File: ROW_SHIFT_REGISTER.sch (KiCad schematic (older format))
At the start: 23 parts, among them Q12 AO3407A, Q13 SSM3K35AMFV, Q14 SSM3K35AMFV, U10 74HC595, U11 74HC595, U12 74HC595, U9 74HC595

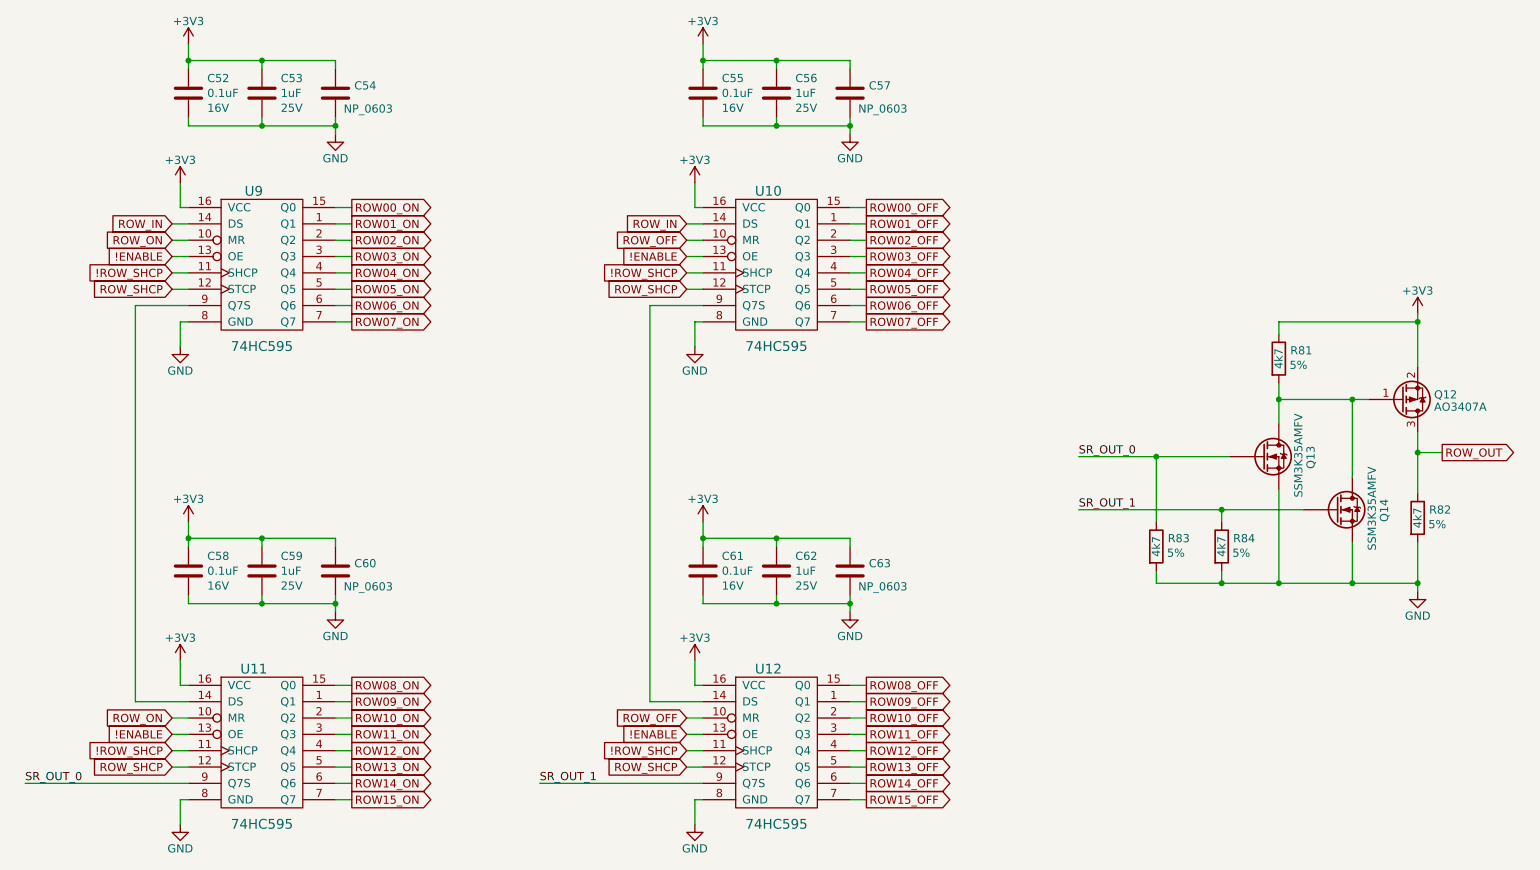
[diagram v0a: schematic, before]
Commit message: automated commit
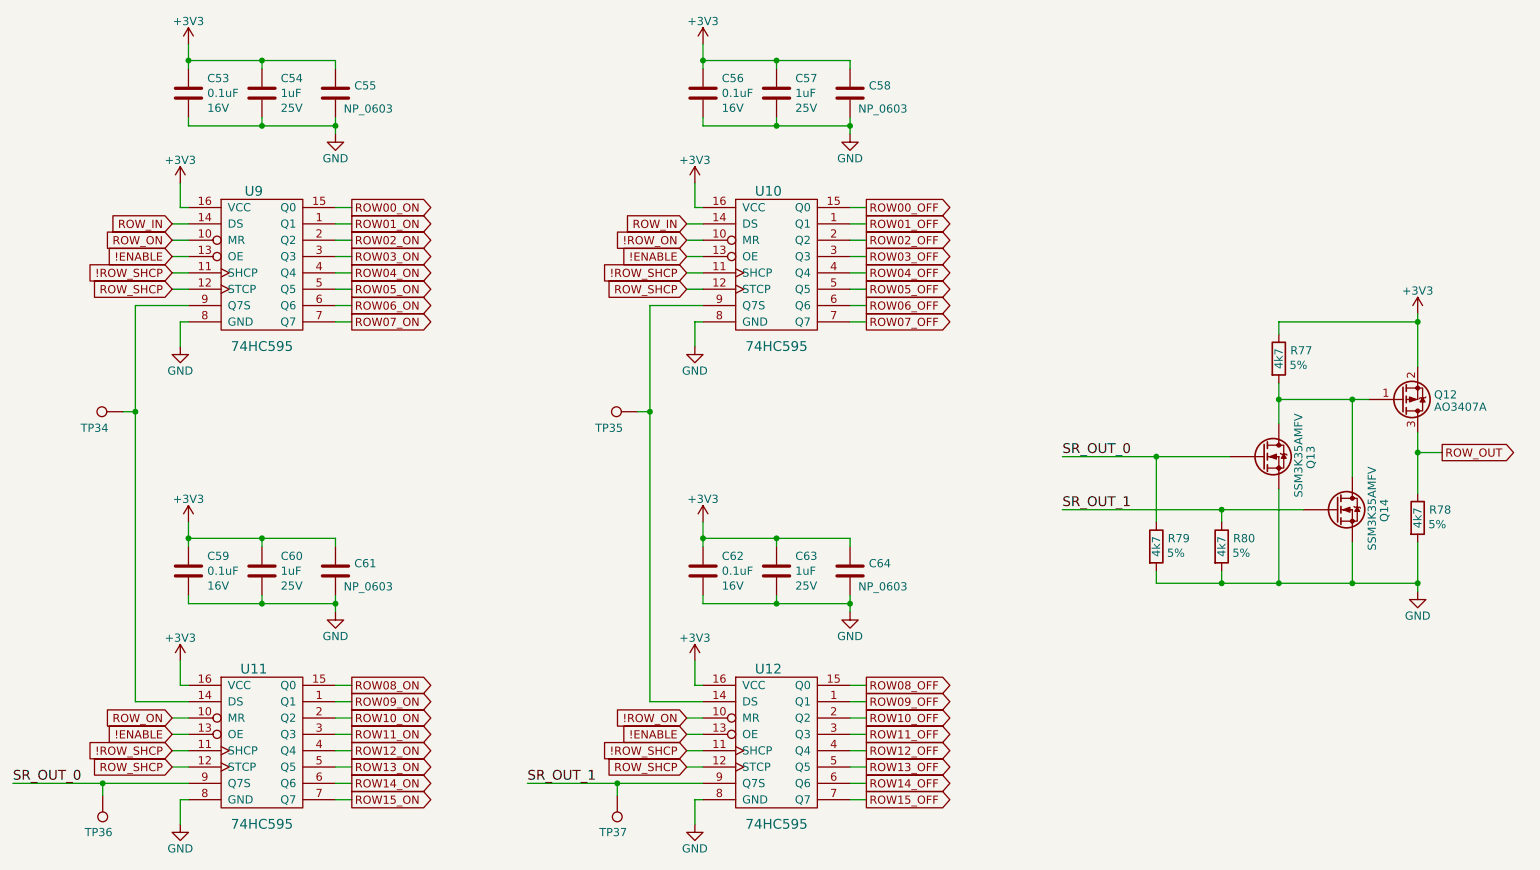
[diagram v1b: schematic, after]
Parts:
- added TP34, TP35, TP36, TP37: TestPoint, symbol Connector:TestPoint
- renumbered C52 to C53, C53 to C54, C54 to C55, C55 to C56, C56 to C57, C57 to C58, C58 to C59, C59 to C60, C60 to C61, C61 to C62, C62 to C63, C63 to C64, R81 to R77, R82 to R78, R83 to R79, R84 to R80
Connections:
- net SR_OUT_0: now also TP36.1
- net SR_OUT_1: now also TP37.1
- net at U11.14 (DS), U9.9 (Q7S): now also TP34.1
- net at U10.9 (Q7S), U12.14 (DS): now also TP35.1
- net ROW_OFF renamed !ROW_ON
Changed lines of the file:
@@
 	1925 2850 1600 2850
 Wire Wire Line
-	1600 2850 1600 5275
+	1600 2850 1600 3500
 Wire Wire Line
 	1600 5275 1925 5275
 Wire Wire Line
-	1925 2350 1825 2350
-Wire Wire Line
 	5025 2100 5025 2250
 Wire Wire Line
@@
 Wire Wire Line
 	5075 2850 4750 2850
-Wire Wire Line
-	4750 2850 4750 5275
 Wire Wire Line
 	4750 5275 5075 5275
@@
 P 2375 1550
 AR Path="/622B9EDC" Ref="C?"  Part="1"
-AR Path="/621F0CB4/622B9EDC" Ref="C53"  Part="1"
-F 0 "C53" H 2490 1641 50  0000 L CNN
+AR Path="/621F0CB4/622B9EDC" Ref="C54"  Part="1"
+F 0 "C54" H 2490 1641 50  0000 L CNN
 F 1 "CL10B105KA8NNNC" H 1425 1100 50  0001 L BNN
 F 2 "Capacitor_SMD:C_0603_1608Metric" H 1425 1000 50  0001 L BNN
@@
 P 1925 1550
 AR Path="/622B9EE4" Ref="C?"  Part="1"
-AR Path="/621F0CB4/622B9EE4" Ref="C52"  Part="1"
-F 0 "C52" H 2040 1641 50  0000 L CNN
+AR Path="/621F0CB4/622B9EE4" Ref="C53"  Part="1"
+F 0 "C53" H 2040 1641 50  0000 L CNN
 F 1 "CL10B104KO8NNNC" H 975 1100 50  0001 L BNN
 F 2 "Capacitor_SMD:C_0603_1608Metric" H 975 1000 50  0001 L BNN
@@
 P 2825 1550
 AR Path="/622B9EEB" Ref="C?"  Part="1"
-AR Path="/621F0CB4/622B9EEB" Ref="C54"  Part="1"
-F 0 "C54" H 2940 1596 50  0000 L CNN
+AR Path="/621F0CB4/622B9EEB" Ref="C55"  Part="1"
+F 0 "C55" H 2940 1596 50  0000 L CNN
 F 1 "NP_0603" H 2875 1425 50  0000 L BNN
 F 2 "Capacitor_SMD:C_0603_1608Metric" H 1875 1000 50  0001 L BNN
@@
 P 2375 4475
 AR Path="/622B9F13" Ref="C?"  Part="1"
-AR Path="/621F0CB4/622B9F13" Ref="C59"  Part="1"
-F 0 "C59" H 2490 4566 50  0000 L CNN
+AR Path="/621F0CB4/622B9F13" Ref="C60"  Part="1"
+F 0 "C60" H 2490 4566 50  0000 L CNN
 F 1 "CL10B105KA8NNNC" H 1425 4025 50  0001 L BNN
 F 2 "Capacitor_SMD:C_0603_1608Metric" H 1425 3925 50  0001 L BNN
@@
 P 1925 4475
 AR Path="/622B9F1B" Ref="C?"  Part="1"
-AR Path="/621F0CB4/622B9F1B" Ref="C58"  Part="1"
-F 0 "C58" H 2040 4566 50  0000 L CNN
+AR Path="/621F0CB4/622B9F1B" Ref="C59"  Part="1"
+F 0 "C59" H 2040 4566 50  0000 L CNN
 F 1 "CL10B104KO8NNNC" H 975 4025 50  0001 L BNN
 F 2 "Capacitor_SMD:C_0603_1608Metric" H 975 3925 50  0001 L BNN
@@
 P 5525 1550
 AR Path="/622B9F4A" Ref="C?"  Part="1"
-AR Path="/621F0CB4/622B9F4A" Ref="C56"  Part="1"
-F 0 "C56" H 5640 1641 50  0000 L CNN
+AR Path="/621F0CB4/622B9F4A" Ref="C57"  Part="1"
+F 0 "C57" H 5640 1641 50  0000 L CNN
 F 1 "CL10B105KA8NNNC" H 4575 1100 50  0001 L BNN
 F 2 "Capacitor_SMD:C_0603_1608Metric" H 4575 1000 50  0001 L BNN
@@
 P 5075 1550
 AR Path="/622B9F52" Ref="C?"  Part="1"
-AR Path="/621F0CB4/622B9F52" Ref="C55"  Part="1"
-F 0 "C55" H 5190 1641 50  0000 L CNN
+AR Path="/621F0CB4/622B9F52" Ref="C56"  Part="1"
+F 0 "C56" H 5190 1641 50  0000 L CNN
 F 1 "CL10B104KO8NNNC" H 4125 1100 50  0001 L BNN
 F 2 "Capacitor_SMD:C_0603_1608Metric" H 4125 1000 50  0001 L BNN
@@
 P 5525 4475
 AR Path="/622B9F81" Ref="C?"  Part="1"
-AR Path="/621F0CB4/622B9F81" Ref="C62"  Part="1"
-F 0 "C62" H 5640 4566 50  0000 L CNN
+AR Path="/621F0CB4/622B9F81" Ref="C63"  Part="1"
+F 0 "C63" H 5640 4566 50  0000 L CNN
 F 1 "CL10B105KA8NNNC" H 4575 4025 50  0001 L BNN
 F 2 "Capacitor_SMD:C_0603_1608Metric" H 4575 3925 50  0001 L BNN
@@
 P 5075 4475
 AR Path="/622B9F89" Ref="C?"  Part="1"
-AR Path="/621F0CB4/622B9F89" Ref="C61"  Part="1"
-F 0 "C61" H 5190 4566 50  0000 L CNN
+AR Path="/621F0CB4/622B9F89" Ref="C62"  Part="1"
+F 0 "C62" H 5190 4566 50  0000 L CNN
 F 1 "CL10B104KO8NNNC" H 4125 4025 50  0001 L BNN
 F 2 "Capacitor_SMD:C_0603_1608Metric" H 4125 3925 50  0001 L BNN
@@
 ROW_ON
 Text GLabel 4975 2450 0    50   Input ~ 0
-ROW_OFF
+!ROW_ON
 Text GLabel 4975 5375 0    50   Input ~ 0
-ROW_OFF
-Text Label 925  5775 0    50   ~ 0
+!ROW_ON
+Text Label 850  5775 0    60   ~ 0
 SR_OUT_0
-Wire Wire Line
-	925  5775 1925 5775
-Text Label 4075 5775 0    50   ~ 0
+Text Label 4000 5775 0    60   ~ 0
 SR_OUT_1
-Wire Wire Line
-	4075 5775 5075 5775
 $Comp
 L custom:SSM3K35AMFV Q?
@@
 	1    0    0    -1
 $EndComp
-Text Label 7375 4100 0    50   ~ 0
+Text Label 7275 4100 0    60   ~ 0
 SR_OUT_1
-Text Label 7375 3775 0    50   ~ 0
+Text Label 7275 3775 0    60   ~ 0
 SR_OUT_0
 Wire Wire Line
-	7375 3775 7850 3775
-$Comp
-L custom:CRG0603F4K7 R83
+	7275 3775 7850 3775
+$Comp
+L custom:CRG0603F4K7 R79
 U 1 1 5D1EAA64
 P 7850 4325
-F 0 "R83" H 7920 4345 50  0000 L BNN
+F 0 "R79" H 7920 4345 50  0000 L BNN
 F 1 "CRG0603F4K7" H 7150 3925 50  0001 L BNN
 F 2 "Resistor_SMD:R_0603_1608Metric" H 7150 3825 50  0001 L BNN
@@
 $EndComp
 $Comp
-L custom:CRG0603F4K7 R84
+L custom:CRG0603F4K7 R80
 U 1 1 5D1EB3B5
 P 8250 4325
-F 0 "R84" H 8320 4345 50  0000 L BNN
+F 0 "R80" H 8320 4345 50  0000 L BNN
 F 1 "CRG0603F4K7" H 7550 3925 50  0001 L BNN
 F 2 "Resistor_SMD:R_0603_1608Metric" H 7550 3825 50  0001 L BNN
@@
 	8600 4550 9050 4550
 $Comp
-L custom:CRG0603F4K7 R81
+L custom:CRG0603F4K7 R77
 U 1 1 5D2191D0
 P 8600 3175
-F 0 "R81" H 8670 3195 50  0000 L BNN
+F 0 "R77" H 8670 3195 50  0000 L BNN
 F 1 "CRG0603F4K7" H 7900 2775 50  0001 L BNN
 F 2 "Resistor_SMD:R_0603_1608Metric" H 7900 2675 50  0001 L BNN
@@
 	9050 3425 8600 3425
 $Comp
-L custom:CRG0603F4K7 R82
+L custom:CRG0603F4K7 R78
 U 1 1 5D22CE7A
 P 9450 4150
-F 0 "R82" H 9520 4170 50  0000 L BNN
+F 0 "R78" H 9520 4170 50  0000 L BNN
 F 1 "CRG0603F4K7" H 8750 3750 50  0001 L BNN
 F 2 "Resistor_SMD:R_0603_1608Metric" H 8750 3650 50  0001 L BNN
@@
 	7850 3775 8300 3775
 Wire Wire Line
-	7375 4100 8250 4100
+	7275 4100 8250 4100
 Wire Wire Line
 	7850 4550 8250 4550
@@
 P 2825 4475
 AR Path="/5D052A90" Ref="C?"  Part="1"
-AR Path="/621F0CB4/5D052A90" Ref="C60"  Part="1"
-F 0 "C60" H 2940 4521 50  0000 L CNN
+AR Path="/621F0CB4/5D052A90" Ref="C61"  Part="1"
+F 0 "C61" H 2940 4521 50  0000 L CNN
 F 1 "NP_0603" H 2875 4350 50  0000 L BNN
 F 2 "Capacitor_SMD:C_0603_1608Metric" H 1875 3925 50  0001 L BNN
@@
 P 5975 4475
 AR Path="/5D053185" Ref="C?"  Part="1"
-AR Path="/621F0CB4/5D053185" Ref="C63"  Part="1"
-F 0 "C63" H 6090 4521 50  0000 L CNN
+AR Path="/621F0CB4/5D053185" Ref="C64"  Part="1"
+F 0 "C64" H 6090 4521 50  0000 L CNN
 F 1 "NP_0603" H 6025 4350 50  0000 L BNN
 F 2 "Capacitor_SMD:C_0603_1608Metric" H 5025 3925 50  0001 L BNN
@@
 P 5975 1550
 AR Path="/5D053792" Ref="C?"  Part="1"
-AR Path="/621F0CB4/5D053792" Ref="C57"  Part="1"
-F 0 "C57" H 6090 1596 50  0000 L CNN
+AR Path="/621F0CB4/5D053792" Ref="C58"  Part="1"
+F 0 "C58" H 6090 1596 50  0000 L CNN
 F 1 "NP_0603" H 6025 1425 50  0000 L BNN
 F 2 "Capacitor_SMD:C_0603_1608Metric" H 5025 1000 50  0001 L BNN
@@
 	1    0    0    -1
 $EndComp
+Wire Wire Line
+	1525 3500 1600 3500
+$Comp
+L Connector:TestPoint TP?
+U 1 1 5D6F7153
+P 1525 3500
+AR Path="/5D6F7153" Ref="TP?"  Part="1"
+AR Path="/61C6D021/5D6F7153" Ref="TP?"  Part="1"
+AR Path="/609E0ED6/5D6F7153" Ref="TP?"  Part="1"
+AR Path="/621F0CB4/5D6F7153" Ref="TP34"  Part="1"
+F 0 "TP34" V 1425 3675 50  0000 C CNN
+F 1 "TestPoint" H 1275 3550 50  0001 C CNN
+F 2 "" H 1725 3500 50  0001 C CNN
+F 3 "~" H 1725 3500 50  0001 C CNN
+	1    1525 3500
+	0    -1   -1   0
+$EndComp
+Connection ~ 1600 3500
+Wire Wire Line
+	1600 3500 1600 5275
+Wire Wire Line
+	4750 2850 4750 3500
+Wire Wire Line
+	4675 3500 4750 3500
+$Comp
+L Connector:TestPoint TP?
+U 1 1 5D702E1C
+P 4675 3500
+AR Path="/5D702E1C" Ref="TP?"  Part="1"
+AR Path="/61C6D021/5D702E1C" Ref="TP?"  Part="1"
+AR Path="/609E0ED6/5D702E1C" Ref="TP?"  Part="1"
+AR Path="/621F0CB4/5D702E1C" Ref="TP35"  Part="1"
+F 0 "TP35" V 4575 3675 50  0000 C CNN
+F 1 "TestPoint" H 4425 3550 50  0001 C CNN
+F 2 "" H 4875 3500 50  0001 C CNN
+F 3 "~" H 4875 3500 50  0001 C CNN
+	1    4675 3500
+	0    -1   -1   0
+$EndComp
+Connection ~ 4750 3500
+Wire Wire Line
+	4750 3500 4750 5275
+Wire Wire Line
+	4000 5775 4550 5775
+Wire Wire Line
+	850  5775 1400 5775
+$Comp
+L Connector:TestPoint TP?
+U 1 1 5D723118
+P 1400 5850
+AR Path="/5D723118" Ref="TP?"  Part="1"
+AR Path="/61C6D021/5D723118" Ref="TP?"  Part="1"
+AR Path="/609E0ED6/5D723118" Ref="TP?"  Part="1"
+AR Path="/621F0CB4/5D723118" Ref="TP36"  Part="1"
+F 0 "TP36" H 1425 6075 50  0000 C CNN
+F 1 "TestPoint" H 1150 5900 50  0001 C CNN
+F 2 "" H 1600 5850 50  0001 C CNN
+F 3 "~" H 1600 5850 50  0001 C CNN
+	1    1400 5850
+	-1   0    0    1
+$EndComp
+Wire Wire Line
+	1400 5850 1400 5775
+Connection ~ 1400 5775
+Wire Wire Line
+	1400 5775 1925 5775
+$Comp
+L Connector:TestPoint TP?
+U 1 1 5D72F4B0
+P 4550 5850
+AR Path="/5D72F4B0" Ref="TP?"  Part="1"
+AR Path="/61C6D021/5D72F4B0" Ref="TP?"  Part="1"
+AR Path="/609E0ED6/5D72F4B0" Ref="TP?"  Part="1"
+AR Path="/621F0CB4/5D72F4B0" Ref="TP37"  Part="1"
+F 0 "TP37" H 4575 6075 50  0000 C CNN
+F 1 "TestPoint" H 4300 5900 50  0001 C CNN
+F 2 "" H 4750 5850 50  0001 C CNN
+F 3 "~" H 4750 5850 50  0001 C CNN
+	1    4550 5850
+	-1   0    0    1
+$EndComp
+Wire Wire Line
+	4550 5850 4550 5775
+Connection ~ 4550 5775
+Wire Wire Line
+	4550 5775 5075 5775
+Wire Wire Line
+	1825 2350 1925 2350
 $EndSCHEMATC

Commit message: automated commit
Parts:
- Q13, Q14: footprint (none) -> Package_TO_SOT_SMD:SOT-723
- U10, U11, U12, U9: footprint (none) -> Package_SO:SOIC-16_3.9x9.9mm_P1.27mm
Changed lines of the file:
@@
 F 0 "U9" H 2325 3050 60  0000 C CNN
 F 1 "74HC595" H 2375 2100 60  0000 C CNN
-F 2 "" H 2075 2650 60  0001 C CNN
-F 3 "" H 2075 2650 60  0001 C CNN
+F 2 "Package_SO:SOIC-16_3.9x9.9mm_P1.27mm" H 2075 2650 60  0001 C CNN
+F 3 "~/datasheets/74HC_HCT595.pdf" H 2075 2650 60  0001 C CNN
 	1    2375 2600
 	1    0    0    -1
@@
 F 0 "U11" H 2325 5975 60  0000 C CNN
 F 1 "74HC595" H 2375 5025 60  0000 C CNN
-F 2 "" H 2075 5575 60  0001 C CNN
+F 2 "Package_SO:SOIC-16_3.9x9.9mm_P1.27mm" H 2075 5575 60  0001 C CNN
 F 3 "" H 2075 5575 60  0001 C CNN
 	1    2375 5525
@@
 F 0 "U10" H 5475 3050 60  0000 C CNN
 F 1 "74HC595" H 5525 2100 60  0000 C CNN
-F 2 "" H 5225 2650 60  0001 C CNN
+F 2 "Package_SO:SOIC-16_3.9x9.9mm_P1.27mm" H 5225 2650 60  0001 C CNN
 F 3 "~/datasheets/74HC_HCT595.pdf" H 5225 2650 60  0001 C CNN
 	1    5525 2600
@@
 F 0 "U12" H 5475 5975 60  0000 C CNN
 F 1 "74HC595" H 5525 5025 60  0000 C CNN
-F 2 "" H 5225 5575 60  0001 C CNN
+F 2 "Package_SO:SOIC-16_3.9x9.9mm_P1.27mm" H 5225 5575 60  0001 C CNN
 F 3 "" H 5225 5575 60  0001 C CNN
 	1    5525 5525
@@
 F 0 "Q13" V 8825 3700 50  0000 L BNN
 F 1 "SSM3K35AMFV" V 8750 3525 50  0000 L BNN
-F 2 "" H 8700 3650 50  0001 L BIN
+F 2 "Package_TO_SOT_SMD:SOT-723" H 8700 3650 50  0001 L BIN
 F 3 "datasheets/SSM3K35AMFV.pdf" H 8700 3625 50  0001 L BNN
 	1    8500 3775
@@
 F 0 "Q14" V 9275 4025 50  0000 L BNN
 F 1 "SSM3K35AMFV" V 9200 3850 50  0000 L BNN
-F 2 "" H 9150 3975 50  0001 L BIN
+F 2 "Package_TO_SOT_SMD:SOT-723" H 9150 3975 50  0001 L BIN
 F 3 "datasheets/SSM3K35AMFV.pdf" H 9150 3950 50  0001 L BNN
 	1    8950 4100
